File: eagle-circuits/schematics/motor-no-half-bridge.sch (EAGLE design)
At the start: 3 parts, among them J1 ARDUINO_R3_SHIELD

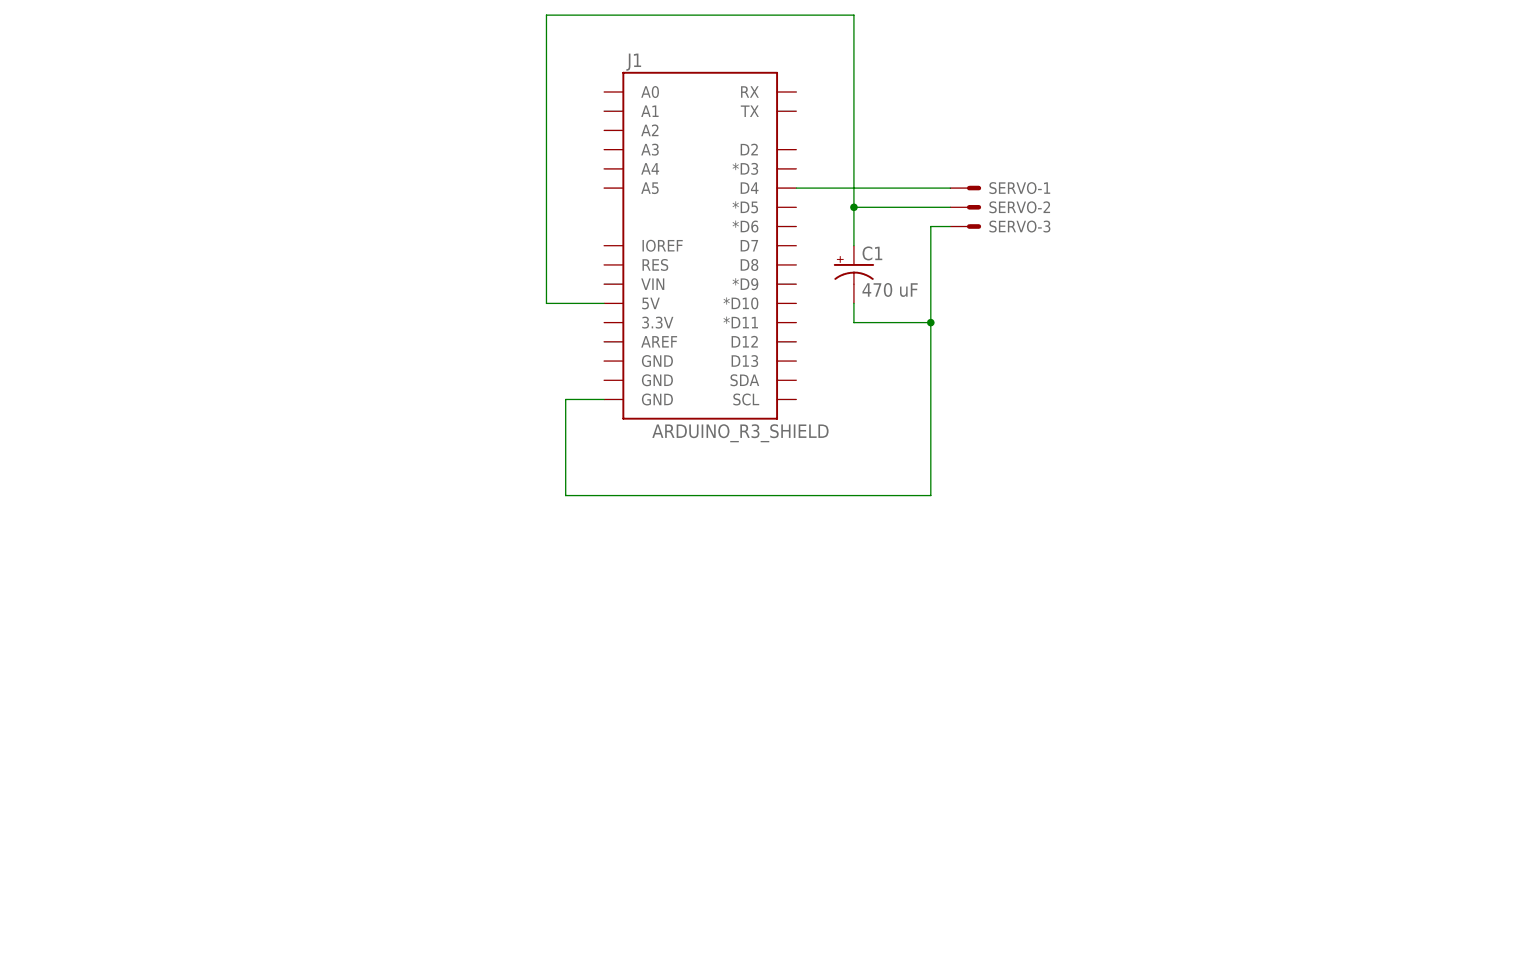
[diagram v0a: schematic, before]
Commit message: added code to src
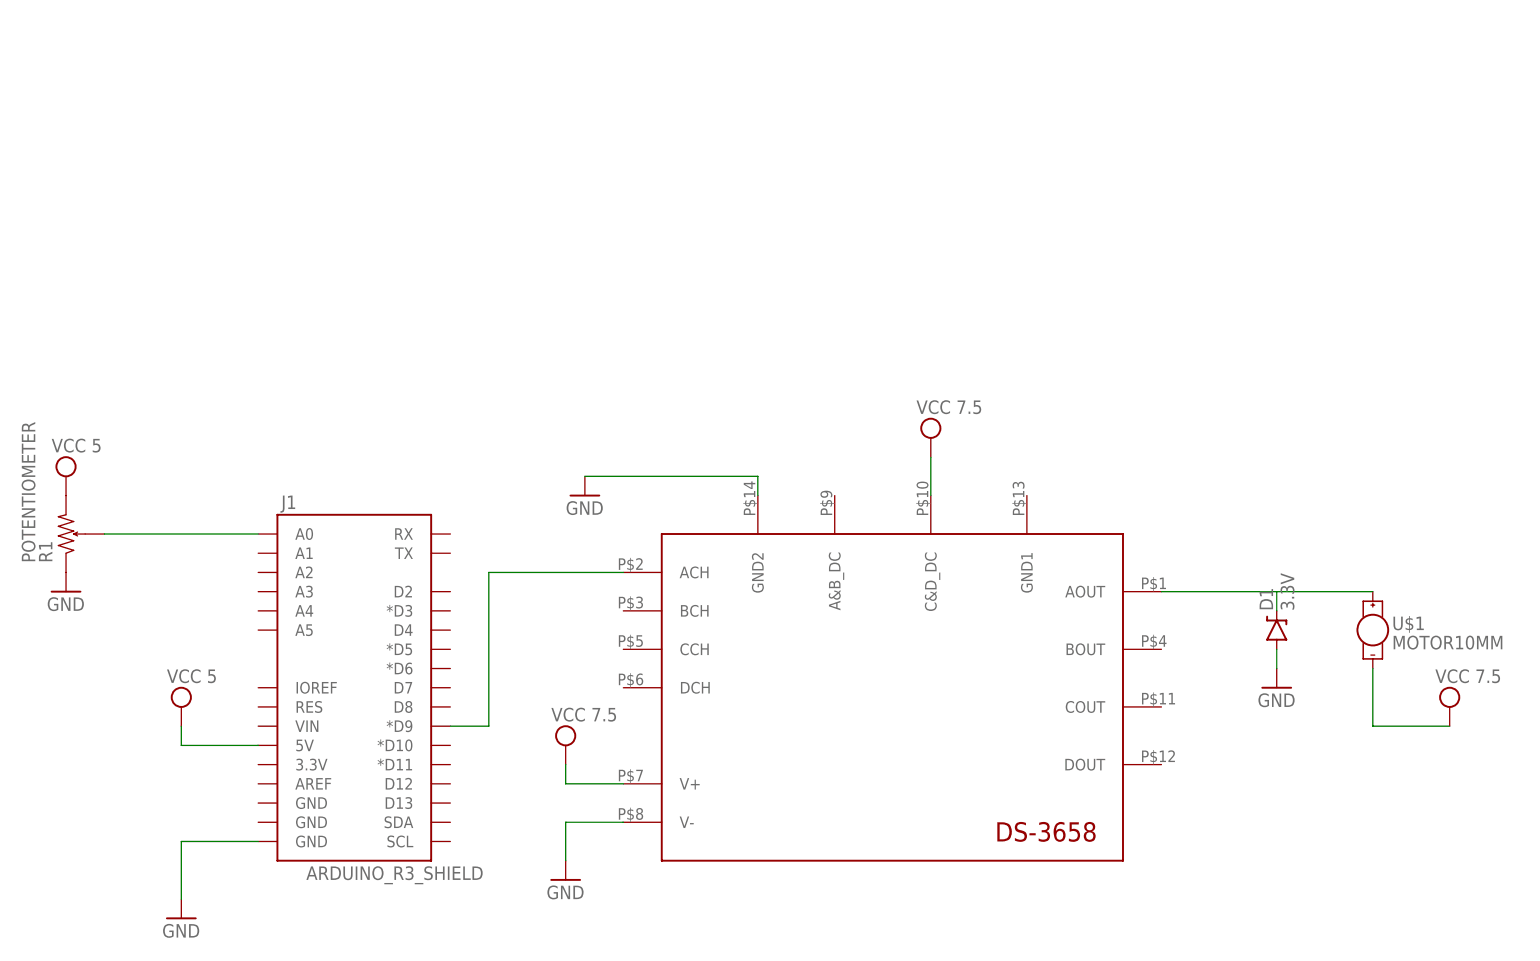
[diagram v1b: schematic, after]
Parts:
- removed C1: 470 uF, ME210Lib_2015_v2:CAP_POL1206
- removed SERVO: 22-23-2031, con-molex:22-23-2031
- added D1: 3.3V, SparkFun-DiscreteSemi:DIODE-ZENER3.3V
- added DS1: DS-3658, me210:DS-3658
- added R1: POTENTIOMETER, SparkFun-Passives:POTENTIOMETER
- added U$1: MOTOR10MM, SparkFun-Electromechanical:MOTOR10MM
- J1: device ME210Lib_2015_v2:ARDUINO_R3_SHIELD -> SparkFun-Boards:ARDUINO_R3_SHIELD
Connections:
- new net GND: DS1.GND2, DS1.V-, J1.GND@0, R1.1
- new net N$4: DS1.ACH, J1.*D9
- new net VCC: DS1.C&D_DC, DS1.V+, J1.5V, R1.2, U$1.-
- net N$1: now also J1.A0, R1.P$1; no longer C1.+, J1.5V, SERVO-2.S
- net N$2: now also D1.C, DS1.AOUT, U$1.+; no longer J1.D4, SERVO-1.S
- net N$3: now also D1.A; no longer C1.-, J1.GND@0, SERVO-3.S
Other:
- moved on the sheet: J1
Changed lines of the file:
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@@
 <layer number="19" name="Unrouted" color="6" fill="1" visible="no" active="no"/>
 <layer number="20" name="Dimension" color="15" fill="1" visible="no" active="no"/>
-<layer number="21" name="tPlace" color="7" fill="1" visible="no" active="no"/>
-<layer number="22" name="bPlace" color="7" fill="1" visible="no" active="no"/>
+<layer number="21" name="tPlace" color="16" fill="1" visible="no" active="no"/>
+<layer number="22" name="bPlace" color="14" fill="1" visible="no" active="no"/>
 <layer number="23" name="tOrigins" color="15" fill="1" visible="no" active="no"/>
 <layer number="24" name="bOrigins" color="15" fill="1" visible="no" active="no"/>
@@
 <layer number="97" name="Info" color="7" fill="1" visible="yes" active="yes"/>
 <layer number="98" name="Guide" color="6" fill="1" visible="yes" active="yes"/>
-<layer number="99" name="SpiceOrder" color="7" fill="1" visible="yes" active="yes"/>
+<layer number="99" name="SpiceOrder" color="7" fill="1" visible="no" active="no"/>
 <layer number="100" name="Muster" color="7" fill="1" visible="no" active="no"/>
 <layer number="101" name="Patch_Top" color="12" fill="4" visible="yes" active="yes"/>
@@
 <layer number="113" name="IDFDebug" color="7" fill="1" visible="yes" active="yes"/>
 <layer number="116" name="Patch_BOT" color="9" fill="4" visible="yes" active="yes"/>
-<layer number="118" name="Rect_Pads" color="7" fill="1" visible="no" active="no"/>
 <layer number="121" name="_tsilk" color="7" fill="1" visible="yes" active="yes"/>
 <layer number="122" name="_bsilk" color="7" fill="1" visible="yes" active="yes"/>
@@
 <layer number="230" name="230bmp" color="7" fill="1" visible="yes" active="yes"/>
 <layer number="231" name="231bmp" color="7" fill="1" visible="yes" active="yes"/>
-<layer number="232" name="Eagle3D_PG2" color="7" fill="1" visible="no" active="no"/>
-<layer number="233" name="Eagle3D_PG3" color="7" fill="1" visible="no" active="no"/>
 <layer number="248" name="Housing" color="7" fill="1" visible="yes" active="yes"/>
 <layer number="249" name="Edge" color="7" fill="1" visible="yes" active="yes"/>
@@
 </classes>
 <parts>
-<part name="FRAME1" library="frames" deviceset="A4L-LOC" device=""/>
-<part name="SERVO" library="con-molex" deviceset="22-23-2031" device="" value=""/>
-<part name="J1" library="ME210Lib_2015_v2" deviceset="ARDUINO_R3_SHIELD" device=""/>
-<part name="C1" library="ME210Lib_2015_v2" deviceset="CAP_POL" device="1206" value="470 uF"/>
+<part name="J1" library="SparkFun-Boards" deviceset="ARDUINO_R3_SHIELD" device=""/>
+<part name="R1" library="SparkFun-Passives" deviceset="POTENTIOMETER" device=""/>
+<part name="SUPPLY1" library="supply2" deviceset="VCC" device="" value="VCC 5"/>
+<part name="GND1" library="supply1" deviceset="GND" device=""/>
+<part name="SUPPLY2" library="supply2" deviceset="VCC" device="" value="VCC 7.5"/>
+<part name="GND2" library="supply1" deviceset="GND" device=""/>
+<part name="SUPPLY3" library="supply2" deviceset="VCC" device="" value="VCC 7.5"/>
+<part name="U$1" library="SparkFun-Electromechanical" deviceset="MOTOR" device="10MM"/>
+<part name="SUPPLY4" library="supply2" deviceset="VCC" device="" value="VCC 7.5"/>
+<part name="GND3" library="supply1" deviceset="GND" device=""/>
+<part name="DS1" library="me210" deviceset="DS-3658" device=""/>
+<part name="GND4" library="supply1" deviceset="GND" device=""/>
+<part name="SUPPLY5" library="supply2" deviceset="VCC" device="" value="VCC 5"/>
+<part name="D1" library="SparkFun-DiscreteSemi" deviceset="DIODE-ZENER" device="3.3V" value="3.3V"/>
+<part name="GND5" library="supply1" deviceset="GND" device=""/>
 </parts>
 <sheets>
@@
 </plain>
 <instances>
-<instance part="FRAME1" gate="G$1" x="0" y="0"/>
-<instance part="SERVO" gate="-1" x="160.02" y="104.14"/>
-<instance part="SERVO" gate="-2" x="160.02" y="101.6"/>
-<instance part="SERVO" gate="-3" x="160.02" y="99.06"/>
-<instance part="J1" gate="G$1" x="124.46" y="99.06"/>
-<instance part="C1" gate="G$1" x="144.78" y="93.98"/>
+<instance part="J1" gate="G$1" x="78.74" y="40.64"/>
+<instance part="R1" gate="G$1" x="40.64" y="58.42" rot="MR90"/>
+<instance part="SUPPLY1" gate="G$1" x="40.64" y="66.04"/>
+<instance part="GND1" gate="1" x="40.64" y="50.8"/>
+<instance part="SUPPLY2" gate="G$1" x="106.68" y="30.48"/>
+<instance part="GND2" gate="1" x="106.68" y="12.7"/>
+<instance part="SUPPLY3" gate="G$1" x="154.94" y="71.12"/>
+<instance part="U$1" gate="G$1" x="213.36" y="45.72"/>
+<instance part="SUPPLY4" gate="G$1" x="223.52" y="35.56"/>
+<instance part="GND3" gate="1" x="55.88" y="7.62"/>
+<instance part="DS1" gate="G$1" x="144.78" y="40.64"/>
+<instance part="GND4" gate="1" x="109.22" y="63.5"/>
+<instance part="SUPPLY5" gate="G$1" x="55.88" y="35.56"/>
+<instance part="D1" gate="G$1" x="200.66" y="45.72" rot="R90"/>
+<instance part="GND5" gate="1" x="200.66" y="38.1"/>
 </instances>
 <busses>
@@
 <net name="N$1" class="0">
 <segment>
-<wire x1="144.78" y1="96.52" x2="144.78" y2="101.6" width="0.1524" layer="91"/>
-<wire x1="144.78" y1="101.6" x2="144.78" y2="127" width="0.1524" layer="91"/>
-<wire x1="144.78" y1="127" x2="104.14" y2="127" width="0.1524" layer="91"/>
-<wire x1="104.14" y1="127" x2="104.14" y2="88.9" width="0.1524" layer="91"/>
+<pinref part="J1" gate="G$1" pin="A0"/>
+<wire x1="66.04" y1="58.42" x2="45.72" y2="58.42" width="0.1524" layer="91"/>
+<pinref part="R1" gate="G$1" pin="P$1"/>
+</segment>
+</net>
+<net name="VCC" class="0">
+<segment>
+<pinref part="R1" gate="G$1" pin="2"/>
+<pinref part="SUPPLY1" gate="G$1" pin="VCC"/>
+</segment>
+<segment>
+<pinref part="SUPPLY2" gate="G$1" pin="VCC"/>
+<wire x1="106.68" y1="27.94" x2="106.68" y2="25.4" width="0.1524" layer="91"/>
+<wire x1="106.68" y1="25.4" x2="114.3" y2="25.4" width="0.1524" layer="91"/>
+<pinref part="DS1" gate="G$1" pin="V+"/>
+</segment>
+<segment>
+<wire x1="154.94" y1="63.5" x2="154.94" y2="68.58" width="0.1524" layer="91"/>
+<pinref part="SUPPLY3" gate="G$1" pin="VCC"/>
+<pinref part="DS1" gate="G$1" pin="C&amp;D_DC"/>
+</segment>
+<segment>
+<pinref part="U$1" gate="G$1" pin="-"/>
+<wire x1="213.36" y1="40.64" x2="213.36" y2="33.02" width="0.1524" layer="91"/>
+<wire x1="213.36" y1="33.02" x2="223.52" y2="33.02" width="0.1524" layer="91"/>
+<pinref part="SUPPLY4" gate="G$1" pin="VCC"/>
+</segment>
+<segment>
 <pinref part="J1" gate="G$1" pin="5V"/>
-<wire x1="104.14" y1="88.9" x2="111.76" y2="88.9" width="0.1524" layer="91"/>
-<pinref part="C1" gate="G$1" pin="+"/>
-<pinref part="SERVO" gate="-2" pin="S"/>
-<wire x1="157.48" y1="101.6" x2="144.78" y2="101.6" width="0.1524" layer="91"/>
-<junction x="144.78" y="101.6"/>
+<wire x1="66.04" y1="30.48" x2="55.88" y2="30.48" width="0.1524" layer="91"/>
+<wire x1="55.88" y1="30.48" x2="55.88" y2="33.02" width="0.1524" layer="91"/>
+<pinref part="SUPPLY5" gate="G$1" pin="VCC"/>
+</segment>
+</net>
+<net name="GND" class="0">
+<segment>
+<pinref part="R1" gate="G$1" pin="1"/>
+<pinref part="GND1" gate="1" pin="GND"/>
+</segment>
+<segment>
+<wire x1="114.3" y1="20.32" x2="106.68" y2="20.32" width="0.1524" layer="91"/>
+<wire x1="106.68" y1="20.32" x2="106.68" y2="15.24" width="0.1524" layer="91"/>
+<pinref part="GND2" gate="1" pin="GND"/>
+<pinref part="DS1" gate="G$1" pin="V-"/>
+</segment>
+<segment>
+<pinref part="J1" gate="G$1" pin="GND@0"/>
+<wire x1="66.04" y1="17.78" x2="55.88" y2="17.78" width="0.1524" layer="91"/>
+<wire x1="55.88" y1="17.78" x2="55.88" y2="10.16" width="0.1524" layer="91"/>
+<pinref part="GND3" gate="1" pin="GND"/>
+</segment>
+<segment>
+<pinref part="DS1" gate="G$1" pin="GND2"/>
+<wire x1="132.08" y1="63.5" x2="132.08" y2="66.04" width="0.1524" layer="91"/>
+<wire x1="132.08" y1="66.04" x2="109.22" y2="66.04" width="0.1524" layer="91"/>
+<pinref part="GND4" gate="1" pin="GND"/>
+</segment>
+</net>
+<net name="N$4" class="0">
+<segment>
+<wire x1="114.3" y1="53.34" x2="96.52" y2="53.34" width="0.1524" layer="91"/>
+<wire x1="96.52" y1="53.34" x2="96.52" y2="33.02" width="0.1524" layer="91"/>
+<pinref part="J1" gate="G$1" pin="*D9"/>
+<wire x1="96.52" y1="33.02" x2="91.44" y2="33.02" width="0.1524" layer="91"/>
+<pinref part="DS1" gate="G$1" pin="ACH"/>
+</segment>
+</net>
+<net name="N$2" class="0">
+<segment>
+<pinref part="DS1" gate="G$1" pin="AOUT"/>
+<wire x1="185.42" y1="50.8" x2="200.66" y2="50.8" width="0.1524" layer="91"/>
+<pinref part="D1" gate="G$1" pin="C"/>
+<wire x1="200.66" y1="50.8" x2="200.66" y2="48.26" width="0.1524" layer="91"/>
+<pinref part="U$1" gate="G$1" pin="+"/>
+<wire x1="200.66" y1="50.8" x2="213.36" y2="50.8" width="0.1524" layer="91"/>
 </segment>
 </net>
 <net name="N$3" class="0">
 <segment>
-<pinref part="SERVO" gate="-3" pin="S"/>
-<wire x1="157.48" y1="99.06" x2="154.94" y2="99.06" width="0.1524" layer="91"/>
-<wire x1="154.94" y1="99.06" x2="154.94" y2="86.36" width="0.1524" layer="91"/>
-<wire x1="154.94" y1="86.36" x2="154.94" y2="63.5" width="0.1524" layer="91"/>
-<wire x1="154.94" y1="63.5" x2="106.68" y2="63.5" width="0.1524" layer="91"/>
-<wire x1="106.68" y1="63.5" x2="106.68" y2="76.2" width="0.1524" layer="91"/>
-<pinref part="J1" gate="G$1" pin="GND@0"/>
-<wire x1="106.68" y1="76.2" x2="111.76" y2="76.2" width="0.1524" layer="91"/>
-<pinref part="C1" gate="G$1" pin="-"/>
-<wire x1="144.78" y1="88.9" x2="144.78" y2="86.36" width="0.1524" layer="91"/>
-<wire x1="144.78" y1="86.36" x2="154.94" y2="86.36" width="0.1524" layer="91"/>
-<junction x="154.94" y="86.36"/>
-</segment>
-</net>
-<net name="N$2" class="0">
-<segment>
-<pinref part="SERVO" gate="-1" pin="S"/>
-<pinref part="J1" gate="G$1" pin="D4"/>
-<wire x1="157.48" y1="104.14" x2="137.16" y2="104.14" width="0.1524" layer="91"/>
-</segment>
-</net>
+<pinref part="D1" gate="G$1" pin="A"/>
+<wire x1="200.66" y1="43.18" x2="200.66" y2="40.64" width="0.1524" layer="91"/>
+<pinref part="GND5" gate="1" pin="GND"/>
+</segment>
+</net>
